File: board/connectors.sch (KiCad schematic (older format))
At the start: 5 parts, among them J3 Conn_ARM_JTAG_SWD_10

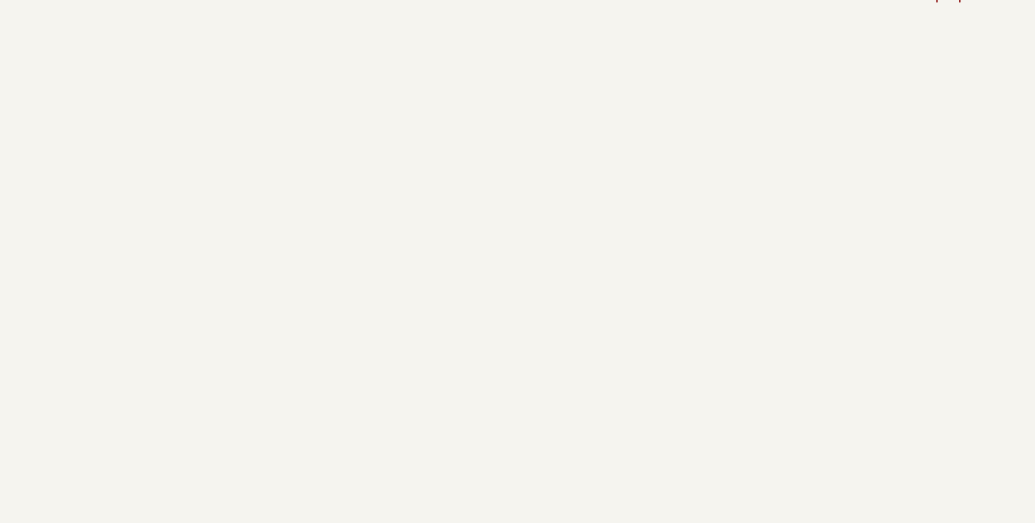
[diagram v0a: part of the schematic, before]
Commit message: Update
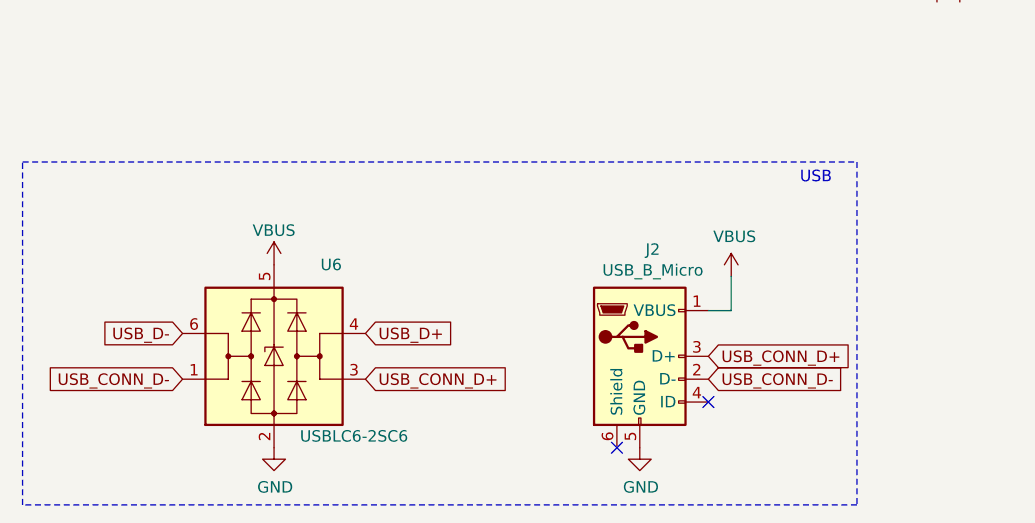
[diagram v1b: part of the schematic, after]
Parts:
- added J2: USB_B_Micro, Connector_USB:USB_Micro-B_Amphenol_10103594-0001LF_Horizontal, symbol board-rescue:USB_B_Micro-Connector
- added U6: USBLC6-2SC6, Package_TO_SOT_SMD:SOT-23-6, symbol Power_Protection:USBLC6-2SC6
- J3: footprint (none) -> Connector_PinHeader_1.27mm:PinHeader_2x05_P1.27mm_Vertical_SMD
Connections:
- new net GND: J2.5 (GND), U6.2 (GND)
- new net USB_CONN_D+: J2.3 (D+), U6.3 (I/O2)
- new net USB_CONN_D-: J2.2 (D-), U6.1 (I/O1)
- new net USB_D+: U6.4 (I/O2)
- new net USB_D-: U6.6 (I/O1)
- new net VBUS: J2.1 (VBUS), U6.5 (VBUS)
- no-connect marks 0 -> 2
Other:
- note added: "USB"
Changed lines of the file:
@@
 F 0 "J3" H 4757 3296 50  0000 R CNN
 F 1 "Conn_ARM_JTAG_SWD_10" H 4757 3205 50  0000 R CNN
-F 2 "" H 5200 3250 50  0001 C CNN
+F 2 "Connector_PinHeader_1.27mm:PinHeader_2x05_P1.27mm_Vertical_SMD" H 5200 3250 50  0001 C CNN
 F 3 "http://infocenter.arm.com/help/topic/com.arm.doc.ddi0314h/DDI0314H_coresight_components_trm.pdf" V 4850 2000 50  0001 C CNN
 	1    5200 3250
 	1    0    0    -1
 $EndComp
+$Comp
+L board-rescue:USB_B_Micro-Connector J2
+U 1 1 60B231B3
+P 3800 5400
+F 0 "J2" H 3857 5867 50  0000 C CNN
+F 1 "USB_B_Micro" H 3857 5776 50  0000 C CNN
+F 2 "Connector_USB:USB_Micro-B_Amphenol_10103594-0001LF_Horizontal" H 3950 5350 50  0001 C CNN
+F 3 "~" H 3950 5350 50  0001 C CNN
+	1    3800 5400
+	1    0    0    -1
+$EndComp
+$Comp
+L power:GND #PWR041
+U 1 1 60B231B9
+P 3800 5800
+F 0 "#PWR041" H 3800 5550 50  0001 C CNN
+F 1 "GND" H 3805 5627 50  0000 C CNN
+F 2 "" H 3800 5800 50  0001 C CNN
+F 3 "" H 3800 5800 50  0001 C CNN
+	1    3800 5800
+	1    0    0    -1
+$EndComp
+NoConn ~ 3700 5800
+$Comp
+L power:VBUS #PWR042
+U 1 1 60B231C0
+P 4200 5050
+F 0 "#PWR042" H 4200 4900 50  0001 C CNN
+F 1 "VBUS" H 4215 5223 50  0000 C CNN
+F 2 "" H 4200 5050 50  0001 C CNN
+F 3 "" H 4200 5050 50  0001 C CNN
+	1    4200 5050
+	1    0    0    -1
+$EndComp
+Wire Wire Line
+	4200 5050 4200 5200
+Wire Wire Line
+	4200 5200 4100 5200
+Text GLabel 4100 5400 2    50   Input ~ 0
+USB_CONN_D+
+Text GLabel 4100 5500 2    50   Input ~ 0
+USB_CONN_D-
+NoConn ~ 4100 5600
+$Comp
+L Power_Protection:USBLC6-2SC6 U6
+U 1 1 60B231CB
+P 2200 5400
+F 0 "U6" H 2450 5800 50  0000 C CNN
+F 1 "USBLC6-2SC6" H 2550 5050 50  0000 C CNN
+F 2 "Package_TO_SOT_SMD:SOT-23-6" H 2200 4900 50  0001 C CNN
+F 3 "https://www.st.com/resource/en/datasheet/usblc6-2.pdf" H 2400 5750 50  0001 C CNN
+	1    2200 5400
+	1    0    0    -1
+$EndComp
+$Comp
+L power:VBUS #PWR039
+U 1 1 60B231D1
+P 2200 5000
+F 0 "#PWR039" H 2200 4850 50  0001 C CNN
+F 1 "VBUS" H 2200 5150 50  0000 C CNN
+F 2 "" H 2200 5000 50  0001 C CNN
+F 3 "" H 2200 5000 50  0001 C CNN
+	1    2200 5000
+	1    0    0    -1
+$EndComp
+Text GLabel 2600 5300 2    50   Input ~ 0
+USB_D+
+Text GLabel 1800 5300 0    50   Input ~ 0
+USB_D-
+Text GLabel 2600 5500 2    50   Input ~ 0
+USB_CONN_D+
+Text GLabel 1800 5500 0    50   Input ~ 0
+USB_CONN_D-
+$Comp
+L power:GND #PWR040
+U 1 1 60B231DB
+P 2200 5800
+F 0 "#PWR040" H 2200 5550 50  0001 C CNN
+F 1 "GND" H 2205 5627 50  0000 C CNN
+F 2 "" H 2200 5800 50  0001 C CNN
+F 3 "" H 2200 5800 50  0001 C CNN
+	1    2200 5800
+	1    0    0    -1
+$EndComp
+Wire Notes Line
+	4750 6050 1100 6050
+Wire Notes Line
+	1100 6050 1100 4550
+Wire Notes Line
+	1100 4550 4750 4550
+Wire Notes Line
+	4750 4550 4750 6050
+Text Notes 4500 4650 0    50   ~ 0
+USB
 $EndSCHEMATC

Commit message: Generic update
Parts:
- added C27: C_Small, Capacitor_SMD:C_0402_1005Metric, symbol Device:C_Small
- added J4, J5, J?: Conn_01x02_Male, Connector_PinHeader_2.54mm:PinHeader_1x02_P2.54mm_Vertical_SMD_Pin1Right, symbol Connector:Conn_01x02_Male
- added R16, R17, R18, R19, R20: 100, Resistor_SMD:R_0603_1608Metric, symbol Device:R_Small_US
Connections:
- net labels added: +3.3V, SWD_!RESET, SWD_TCK, SWD_TDI, SWD_TDO, SWD_TMS
- wire segments 2 -> 19
- no-connect marks 2 -> 3
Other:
- note added: "12V power in"
- note added: "5V PWR OUT\nGND"
- note added: "Decoupling filter for reset pin ??????\n"
- note added: "Mounting holes\n"
- note added: "SWD\n"
- note added: "USART\n"
- moved on the sheet: H1, H2, H3, H4, J3

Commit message: Updated schematic
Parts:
- removed J4, J5, J?: Conn_01x02_Male, Connector_PinHeader_2.54mm:PinHeader_1x02_P2.54mm_Vertical_SMD_Pin1Right, symbol Connector:Conn_01x02_Male
- removed R17: 100, Resistor_SMD:R_0603_1608Metric, symbol Device:R_Small_US
- added J4: Conn_01x04_Male, symbol Connector:Conn_01x04_Male
- added J5: Screw_Terminal_01x02, symbol Connector:Screw_Terminal_01x02
- C30: renamed from C27; value C_Small -> 100n
- R20: renamed from R19; value 100 -> 10k
- renumbered J3 to J2, J2 to J3, R16 to R18, R18 to R19, R20 to R21
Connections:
- net labels added: +5V, 12V_IN, SWDCLK, SWDIO, SWO, USART3_RX, USART3_TX
- net labels removed: SWD_TCK, SWD_TDI, SWD_TDO, SWD_TMS
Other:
- note added: "Connectors"
- note added: "External Connectors\n"
- note added: "Serial Wire Debug\n"
- note removed: "12V power in"
- note removed: "5V PWR OUT\nGND"
- note removed: "SWD\n"
- note removed: "USART\n"
- moved on the sheet: C30, H1, H2, H3, H4, J2, J3, R18, R19, R20, R21, U6
